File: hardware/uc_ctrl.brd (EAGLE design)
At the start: 28 x 31 mm, 32 parts, among them Q4 si2305cd, Q7 si2305cd, T1 BC846, T3 BC846, Y1 32768Hz CFPX-217 12.5pF

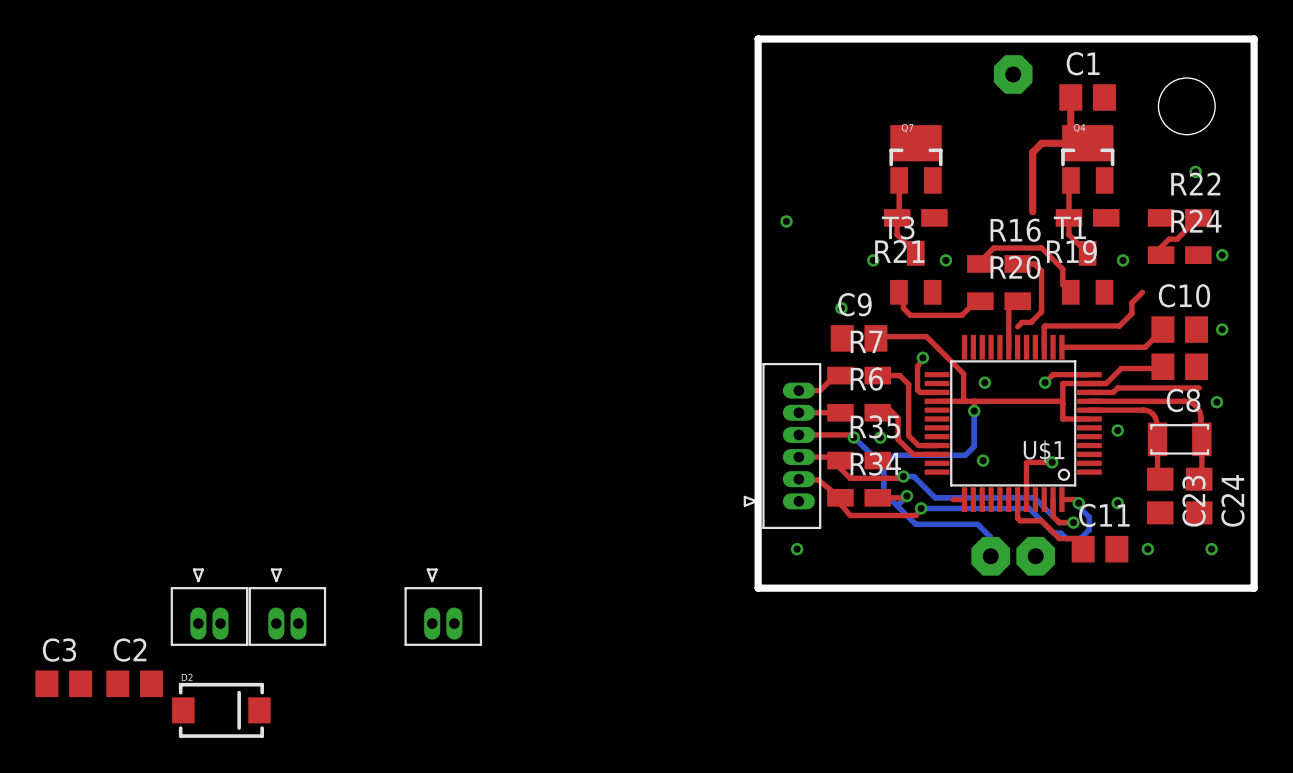
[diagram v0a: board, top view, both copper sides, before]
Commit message: add pcb
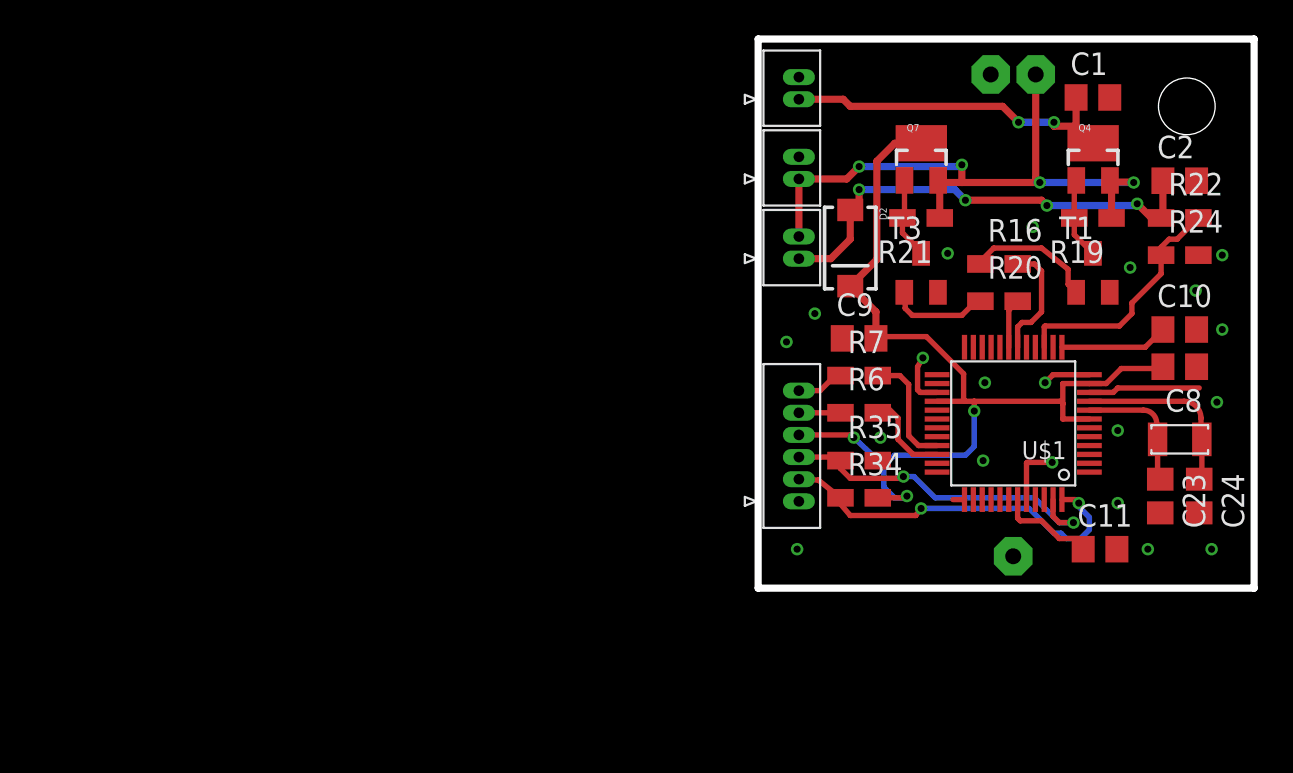
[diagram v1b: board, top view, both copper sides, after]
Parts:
- removed C3: 100nF, rcl:C0805
- moved C2 65.5 mm to (23.8, 23.0)
- moved D2 44.1 mm to (5.20, 19.2), turned to 270 degrees
- moved U$9 39.7 mm to (2.30, 18.6), turned to 90 degrees
- moved U$5 38.7 mm to (2.30, 23.1), turned to 90 degrees
- moved U$3 36.1 mm to (2.30, 27.6), turned to 90 degrees
- moved U$7 30.1 mm to (23.6, 3.10)
- moved Q7 0.30 mm to (9.20, 24.4)
- moved R21 0.30 mm to (9.20, 20.9)
- moved T3 0.30 mm to (9.20, 17.8)
- moved C1 0.30 mm to (18.9, 27.7)
- moved Q4 0.30 mm to (18.9, 24.4)
- moved R19 0.30 mm to (18.9, 20.9)
- moved T1 0.30 mm to (18.9, 17.8)
- turned G1 to 270 degrees
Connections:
- net N$4 renamed UC_POW
- net 3V_CELL: now also U$9.2; no longer U$9.1
- net GND: no longer C3.1
- net PUSH: now also U$9.1; no longer U$9.2
- net UC_EN: now also U$1.18; no longer U$1.19
- net VCC: no longer C3.2
- net VCC_EN: now also U$1.19; no longer U$1.18
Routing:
- net 3V_CELL: track 0.00 -> 36.6 mm, vias 0 -> 4
- net PUSH: track 0.00 -> 26.3 mm, vias 0 -> 4
- net UC_POW: track 9.66 -> 19.4 mm, vias 0 -> 2
- net VCC: track 50.1 -> 56.4 mm
- net VCC_EN: track 0.00 -> 2.81 mm
- net P1.1: track 11.2 -> 13.8 mm
- net UC_EN: track 7.61 -> 6.67 mm
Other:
- board text added: "3Vext"
- board text added: "http://github.com/rodan/ucurrent_ctrl"
- board text added: "rev 1.0 201312"
- board text added: "sw"
- board text added: "uCurrent"
- board text removed: "avp"
- board text removed: "http://github.com/rodan/interphone"
- board text removed: "ip rev 2.0 201312"
- board text removed: "mp"
- board text removed: "px"
